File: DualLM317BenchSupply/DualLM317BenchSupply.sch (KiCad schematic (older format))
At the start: 25 parts, among them CON101 BARREL_JACK, P103 CONN_1, P104 CONN_1, SW101 SPDT, SW102 SPDT, SW103 SPDT, U101 LM317, U102 LM317, U103 7805

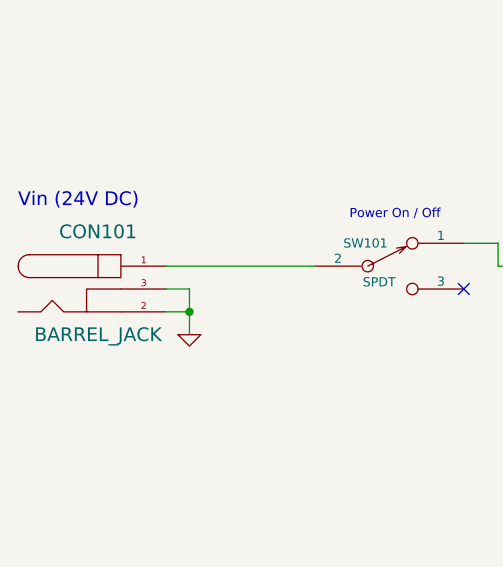
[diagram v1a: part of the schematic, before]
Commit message: updating switch
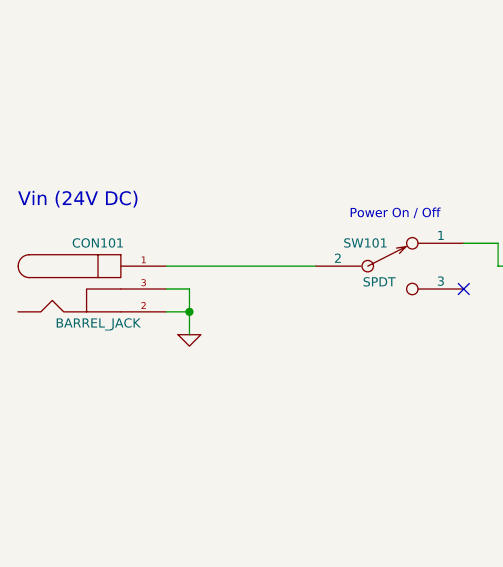
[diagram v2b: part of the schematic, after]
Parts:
- CON101: footprint (none) -> ~
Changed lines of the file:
@@
 EESchema Schematic File Version 2
+LIBS:connectors_PL
 LIBS:displays_PL
 LIBS:resistors_PL
@@
 	5800 6300 5800 4200
 Connection ~ 5800 4200
-$Comp
-L BARREL_JACK CON101
-U 1 1 53267050
-P 2200 4300
-F 0 "CON101" H 2200 4550 60  0000 C CNN
-F 1 "BARREL_JACK" H 2200 4100 60  0000 C CNN
-F 2 "" H 2200 4300 60  0000 C CNN
-F 3 "" H 2200 4300 60  0000 C CNN
-	1    2200 4300
-	1    0    0    -1
-$EndComp
 Wire Wire Line
 	2500 4300 2600 4300
@@
 Wire Wire Line
 	3150 4200 2500 4200
+$Comp
+L BARREL_JACK CON101
+U 1 1 53265EFE
+P 2200 4300
+F 0 "CON101" H 2200 4500 40  0000 C CNN
+F 1 "BARREL_JACK" H 2200 4150 40  0000 C CNN
+F 2 "~" H 2200 4300 60  0000 C CNN
+F 3 "~" H 2200 4300 60  0000 C CNN
+	1    2200 4300
+	1    0    0    -1
+$EndComp
 $EndSCHEMATC
